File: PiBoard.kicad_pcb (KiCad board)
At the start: 4 copper layers, 90.1 x 92.5 mm, 129 parts, among them IC1 TCAN337DCNR, IC2 TPS2557QDRBTQ1, IC3 LM74502HDDFR, IC4 AP64501QSP-13, IC5 TPS2557QDRBTQ1, IC7 TPS2557QDRBTQ1, IC8 TPS2557QDRBTQ1, J1 CarLVPowerConnector, J10 USB_C_Receptacle, J11 RTC Battery Port, J14 4x nano-fit, J2 Display Breakout, J3 2222, J5 USB_C_Receptacle_USB2.0_16P, J6 CarCANConnector, J7 USB_C_Receptacle_USB2.0_16P, J8 CarCANConnector, J9 HDMI_E, Q1 PSMN8R5-40MSDX, SW1 SW_Push, SW2 SW_Push, U13 CDSOT23-T24CAN, U14 MCP2515-E/STVAO, Y4 8 MHz

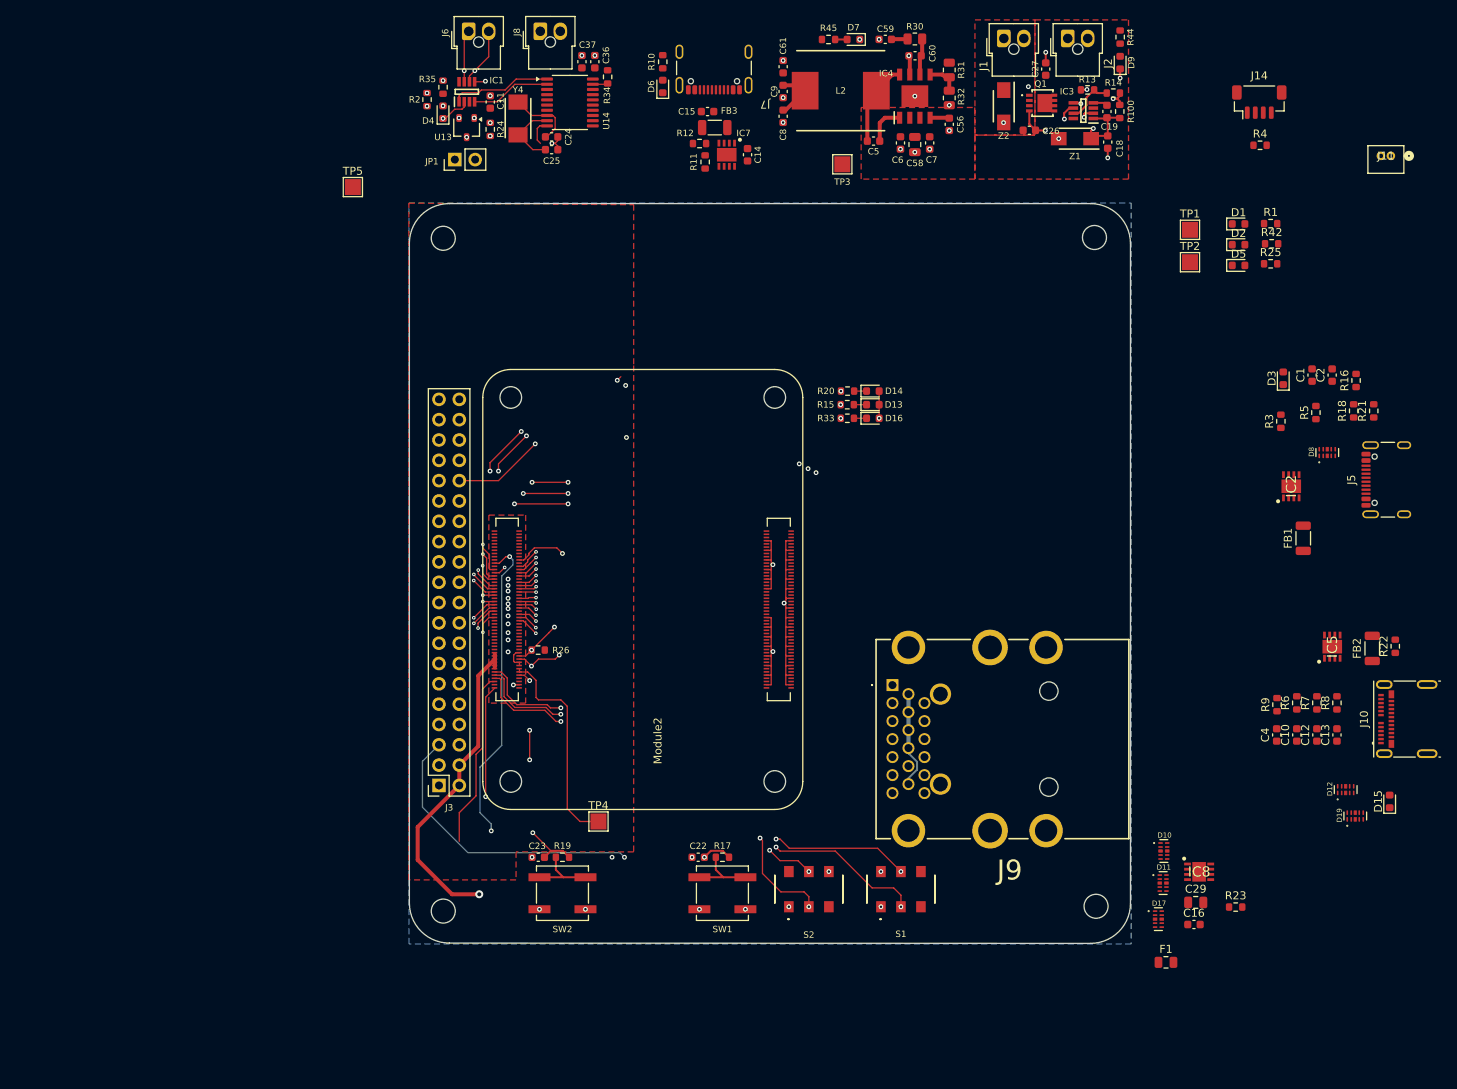
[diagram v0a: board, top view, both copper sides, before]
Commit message: I hate my life
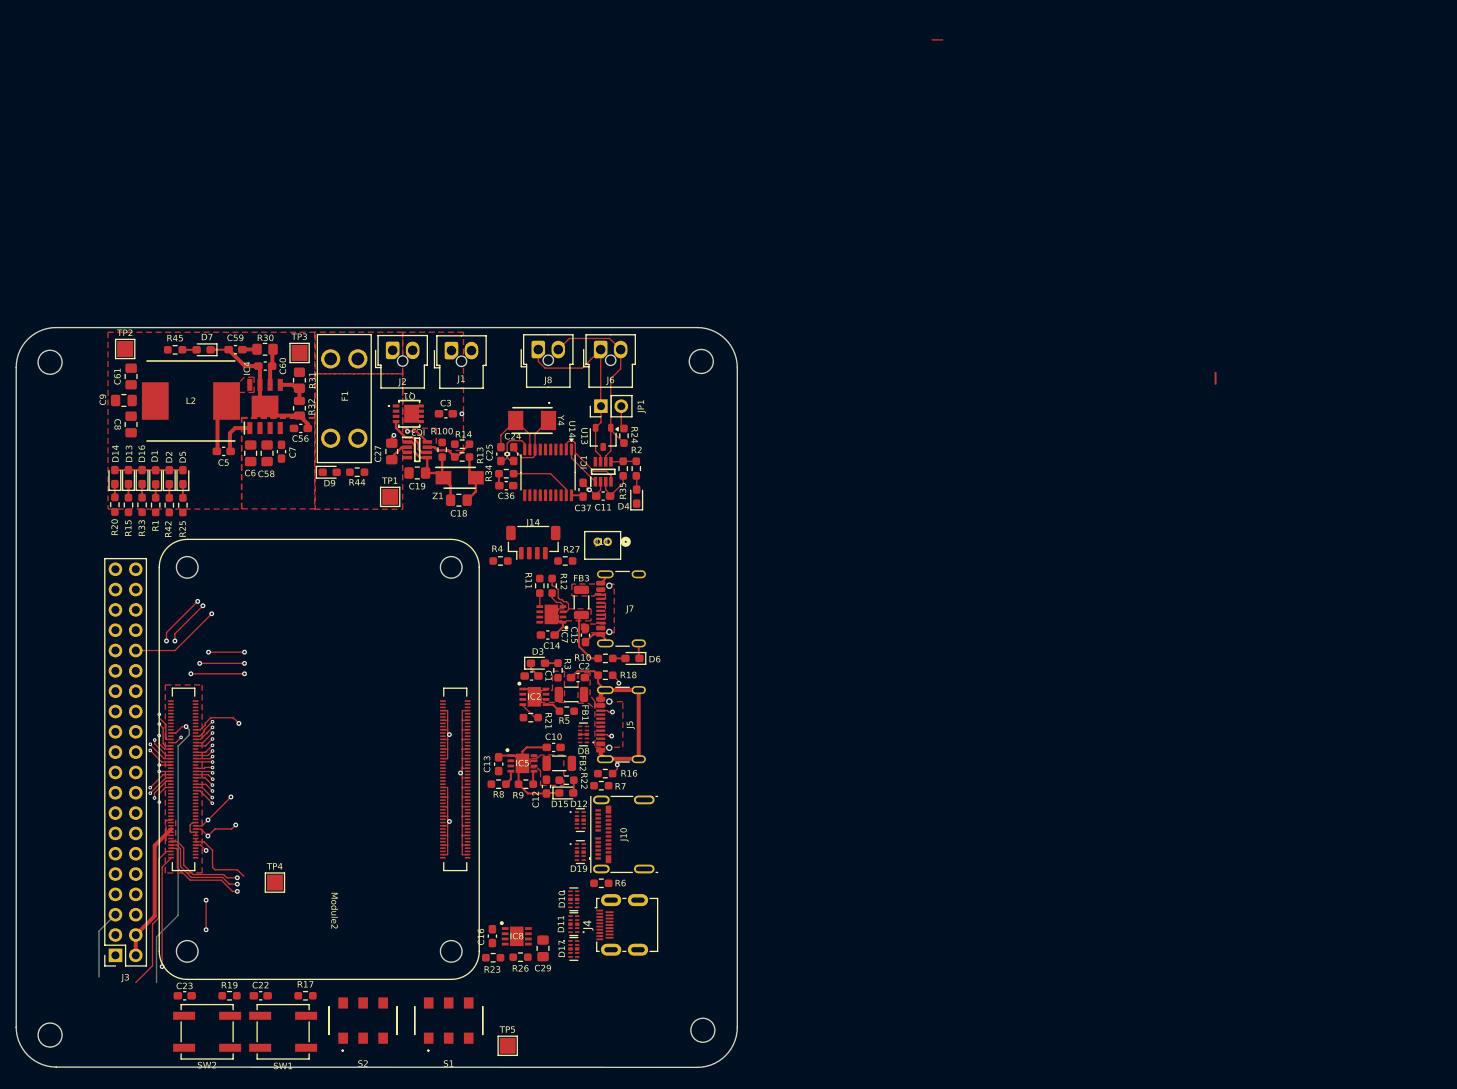
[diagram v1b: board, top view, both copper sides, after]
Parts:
- removed C26: 22n, Capacitor_SMD:C_0603_1608Metric
- removed C4: 120uF, Capacitor_SMD:C_0603_1608Metric
- removed J9: HDMI_E, Controls_Pi:MX50019NQ1
- removed Z2: SMAF4751A-TP, UTSVT_Passives:SODFL5026X125N
- added C3: 0.1u, Capacitor_SMD:C_0603_1608Metric_Pad1.08x0.95mm_HandSolder, F.Cu at (106.3, 77.5)
- added J4: HDMI_D_1.4, Connector_Video:HDMI_Micro-D_Molex_46765-1x01, F.Cu at (130.3, 141.4)
- added R27: 10K, Resistor_SMD:R_0603_1608Metric_Pad0.98x0.95mm_HandSolder, F.Cu at (121.3, 95.9)
- C1, C10, C11, C12, C13, C14, C15, C16, C2, C22, C23, C36, C37, C5, C56, C59, C60, C7: footprint Capacitor_SMD:C_0603_1608Metric -> Capacitor_SMD:C_0603_1608Metric_Pad1.08x0.95mm_HandSolder
- C18, C19, C27, C6, C61, C8, C9: footprint Capacitor_SMD:C_0603_1608Metric -> Capacitor_SMD:C_0805_2012Metric_Pad1.18x1.45mm_HandSolder
- C24, C25: value 26 pF -> 22 pF; footprint Capacitor_SMD:C_0603_1608Metric -> Capacitor_SMD:C_0603_1608Metric_Pad1.08x0.95mm_HandSolder
- C29, C58: footprint Capacitor_SMD:C_0805_2012Metric -> Capacitor_SMD:C_0805_2012Metric_Pad1.18x1.45mm_HandSolder
- D1, D13, D14, D15, D16, D2, D3, D4, D5, D6, D7, D9: footprint LED_SMD:LED_0603_1608Metric -> LED_SMD:LED_0603_1608Metric_Pad1.05x0.95mm_HandSolder
- F1: value 1A -> 3568; footprint Fuse:Fuse_0805_2012Metric -> Controls_Pi:FUSE_3568
- Q1: footprint UTSVT_Power_SP:PSMN8R5-40MSDX -> UTSVT_Power:PSMN8R5-40MSDX
- R1, R42: value 1k -> 700; footprint Resistor_SMD:R_0603_1608Metric -> Resistor_SMD:R_0603_1608Metric_Pad0.98x0.95mm_HandSolder
- R10, R100, R11, R12, R13, R14, R15, R16, R17, R18, R19, R2, R20, R21, R22, R23, R24, R25, R26, R3, R33, R34, R35, R44, R45, R5, R6, R7, R8, R9: footprint Resistor_SMD:R_0603_1608Metric -> Resistor_SMD:R_0603_1608Metric_Pad0.98x0.95mm_HandSolder
- R30, R31: footprint Resistor_SMD:R_0805_2012Metric -> Resistor_SMD:R_0805_2012Metric_Pad1.20x1.40mm_HandSolder
- R4: value 10K 1% -> 10K; footprint Resistor_SMD:R_0603_1608Metric -> Resistor_SMD:R_0603_1608Metric_Pad0.98x0.95mm_HandSolder
- moved R1 143.7 mm to (70.1, 89.0), turned to -90 degrees
- moved R42 141.6 mm to (71.8, 89.0), turned to -90 degrees
- moved R25 139.3 mm to (73.5, 89.0), turned to -90 degrees
- moved D1 139.0 mm to (70.1, 85.5), turned to 90 degrees
- moved D2 136.8 mm to (71.8, 85.5), turned to 90 degrees
- moved D5 134.6 mm to (73.5, 85.5), turned to 90 degrees
- moved TP2 133.5 mm to (66.2, 69.4)
- moved F1 124.6 mm to (93.6, 75.6), turned to -90 degrees
- moved R21 112.1 mm to (116.9, 115.5), turned to 0 degrees
- moved D9 111.3 mm to (91.8, 84.8), turned to 0 degrees
- moved R44 109.8 mm to (95.2, 84.8), turned to 180 degrees
- moved J11 109.1 mm to (126.6, 93.5)
- moved TP5 109.1 mm to (114.1, 156.5)
- moved R4 108.2 mm to (113.2, 95.9), turned to 180 degrees
- moved J14 106.1 mm to (117.3, 93.6)
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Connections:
- D11 pad 1: /High Speed/HDMI0_CK_P -> /High Speed/HDMI0_CK_N
- D11 pad 10: /High Speed/HDMI0_CK_P -> /High Speed/HDMI0_CK_N
- D11 pad 2: /High Speed/HDMI0_CK_N -> /High Speed/HDMI0_CK_P
- D11 pad 4: /High Speed/HDMI0_D1_P -> /High Speed/HDMI0_D1_N
- D11 pad 5: /High Speed/HDMI0_D1_N -> /High Speed/HDMI0_D1_P
- D11 pad 6: /High Speed/HDMI0_D1_N -> /High Speed/HDMI0_D1_P
- D11 pad 7: /High Speed/HDMI0_D1_P -> /High Speed/HDMI0_D1_N
- D11 pad 9: /High Speed/HDMI0_CK_N -> /High Speed/HDMI0_CK_P
- D12 pad 1: /High Speed/USB_HUB_D- -> unconnected-(D12-D1+-Pad1)
- D12 pad 10: /High Speed/USB_HUB_D- -> unconnected-(D12-NC_4-Pad10)
- D12 pad 2: /High Speed/USB_HUB_D+ -> unconnected-(D12-D1--Pad2)
- D12 pad 4: unconnected-(D12-D2+-Pad4) -> /High Speed/USB_HUB_D-
- D12 pad 5: unconnected-(D12-D2--Pad5) -> /High Speed/USB_HUB_D+
- D12 pad 6: unconnected-(D12-NC_1-Pad6) -> /High Speed/USB_HUB_D+
- D12 pad 7: unconnected-(D12-NC_2-Pad7) -> /High Speed/USB_HUB_D-
- D12 pad 9: /High Speed/USB_HUB_D+ -> unconnected-(D12-NC_3-Pad9)
- D17 pad 2: /High Speed/HDMI0_HOTPLUG -> /High Speed/HDMI0_SCL
- D17 pad 4: /High Speed/HDMI0_SCL -> /High Speed/HDMI0_SDA
- D17 pad 5: /High Speed/HDMI0_SDA -> /High Speed/HDMI0_HOTPLUG
- D17 pad 6: /High Speed/HDMI0_SDA -> /High Speed/HDMI0_HOTPLUG
- D17 pad 7: /High Speed/HDMI0_SCL -> /High Speed/HDMI0_SDA
- D17 pad 9: /High Speed/HDMI0_HOTPLUG -> /High Speed/HDMI0_SCL
- D8 pad 1: /High Speed/USB_DBG_D- -> unconnected-(D8-D1+-Pad1)
- D8 pad 10: /High Speed/USB_DBG_D- -> unconnected-(D8-NC_4-Pad10)
- D8 pad 2: /High Speed/USB_DBG_D+ -> unconnected-(D8-D1--Pad2)
- D8 pad 4: unconnected-(D8-D2+-Pad4) -> /High Speed/USB_DBG_D-
- D8 pad 5: unconnected-(D8-D2--Pad5) -> /High Speed/USB_DBG_D+
- D8 pad 6: unconnected-(D8-NC_1-Pad6) -> /High Speed/USB_DBG_D+
- D8 pad 7: unconnected-(D8-NC_2-Pad7) -> /High Speed/USB_DBG_D-
- D8 pad 9: /High Speed/USB_DBG_D+ -> unconnected-(D8-NC_3-Pad9)
- Q1 pad 1: /Power Distribution/LV+ -> +24V
- Q1 pad 10: +24V -> /Power Distribution/LV+
- Q1 pad 11: +24V -> /Power Distribution/LV+
- Q1 pad 2: /Power Distribution/LV+ -> +24V
- Q1 pad 3: /Power Distribution/LV+ -> +24V
- Q1 pad 5: +24V -> /Power Distribution/LV+
- Q1 pad 6: +24V -> /Power Distribution/LV+
- Q1 pad 7: +24V -> /Power Distribution/LV+
- Q1 pad 8: +24V -> /Power Distribution/LV+
- Q1 pad 9: +24V -> /Power Distribution/LV+
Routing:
- net /CM5 GPIO/EEPROM_nWP: track 77.9 -> 8.60 mm, vias 3 -> 1
- net /CM5 GPIO/BT_Disable: track 73.6 -> 11.6 mm, vias 3 -> 1
- net /CM5 GPIO/WiFi_Disable: track 71.8 -> 11.4 mm, vias 3 -> 1
- net /CM5 GPIO/nRPIBOOT: track 59.2 -> 11.8 mm, vias 3 -> 1
- net /CM5 GPIO/GPIO13: track 91.1 -> 50.0 mm, vias 5 -> 3
- net /CM5 GPIO/GPIO19: track 87.5 -> 46.6 mm, vias 5 -> 3
- net /CM5 GPIO/GPIO26: track 84.3 -> 43.6 mm, vias 5 -> 3
- net unconnected-(Module2A-SDA0-Pad82): track 64.7 -> 29.1 mm
- net /CM5 GPIO/PWR_BUTT: track 47.1 -> 12.9 mm, vias 4 -> 3
- net +5V: track 47.0 -> 17.6 mm, vias 1 -> 0
- net /CM5 GPIO/GPIO3: track 79.1 -> 51.3 mm, vias 2 -> 1
- net unconnected-(Module2A-SCL0-Pad80): track 0.00 -> 24.8 mm, vias 0 -> 2
- net +3.3V: track 39.2 -> 19.6 mm, vias 2 -> 0
- net /CM5 GPIO/CAN_SPI_CS: track 43.5 -> 26.1 mm
- net +1.8V: track 26.8 -> 9.40 mm
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- added copper zone on F.Cu, net +5V
- added copper zone on F.Cu, net /High Speed/USB-C/VBUS_DBG
- added copper zone on F.Cu, net /High Speed/USB-C/VBUS_HUB
- added copper zone on F.Cu, net /High Speed/USB-C/VBUS_PWR
- added copper zone on F.Cu, net Net-(C15-Pad1)
- added copper zone on F.Cu, net Net-(C2-Pad1)
- added copper zone on F.Cu, net Net-(IC4-SW)
- added copper zone on F.Cu, net Net-(J2-+24V)
- removed copper zone on F.Cu, net +3.3V
- removed copper zone on B.Cu, net GND
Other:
- board text added: "For Instructional Use Only."
- board text added: "SOLIDWORKS Educational Product."
- board text removed: "Left some of these pwr components 0805 (?)"
- board text removed: "Trying to keep this space more open for fancy routing ig"

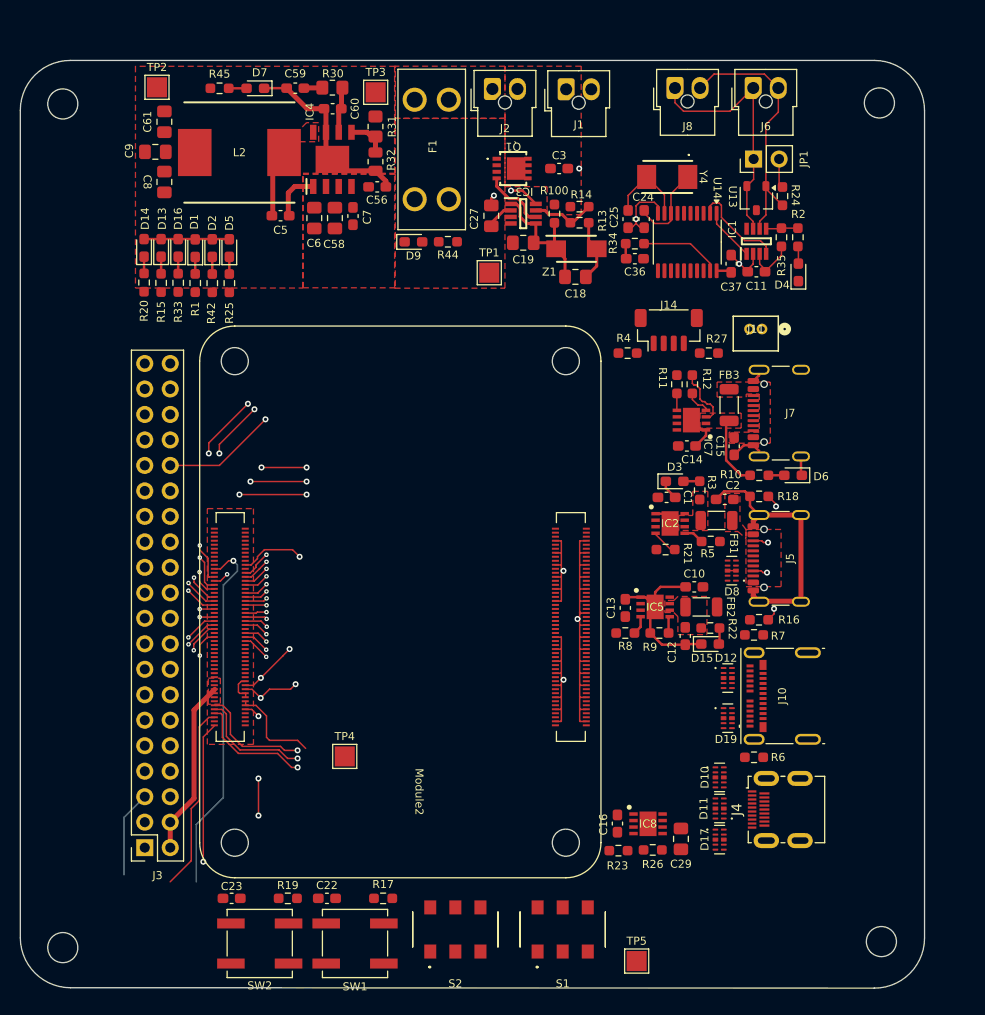
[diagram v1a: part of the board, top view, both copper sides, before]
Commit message: I'm unhappy with the state of the world
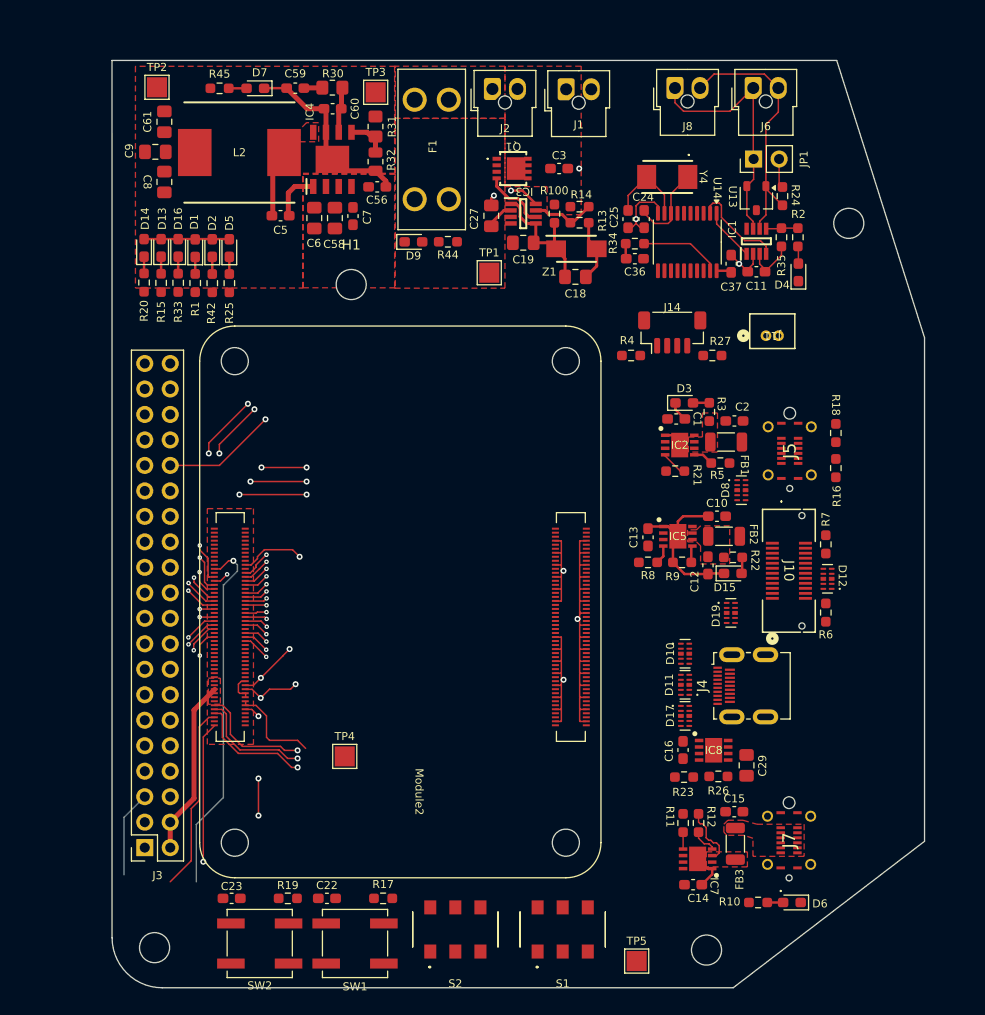
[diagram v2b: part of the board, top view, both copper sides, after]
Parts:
- J10: footprint Connector_USB:USB_C_Receptacle_Molex_105450-0101 -> Controls_Pi:CONN_221608-0001_MOL
- J5: footprint Connector_USB:USB_C_Receptacle_GCT_USB4105-xx-A_16P_TopMnt_Horizontal -> Controls_Pi:2193200001
- J7: footprint UTSVT_Connectors:USB_C_Receptacle_GCT_USB4105-xx-A_16P_TopMnt_Horizontal -> Controls_Pi:2193200001
- moved C14 43.7 mm to (119.7, 148.9)
- moved R11 43.7 mm to (118.7, 142.8)
- moved R12 43.7 mm to (120.2, 142.8)
- moved FB3 43.7 mm to (123.9, 144.8)
- moved IC7 43.7 mm to (120.1, 146.3)
- moved J7 42.6 mm to (129.2, 144.5)
- moved D6 42.6 mm to (129.5, 150.7)
- moved R10 42.6 mm to (126.2, 150.7)
- moved C15 36.4 mm to (123.8, 141.7), turned to 180 degrees
- moved H1 33.9 mm to (85.6, 89.1)
- moved H4 17.5 mm to (121.0, 155.4)
- moved R16 16.9 mm to (133.9, 107.4), turned to 90 degrees
- moved R6 16.1 mm to (132.9, 121.8), turned to -90 degrees
- moved D12 14.0 mm to (133.1, 118.4), turned to 180 degrees
- moved D11 12.8 mm to (118.9, 129.0)
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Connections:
- D8 pad 1: unconnected-(D8-D1+-Pad1) -> /High Speed/USB_DBG_D-
- D8 pad 10: unconnected-(D8-NC_4-Pad10) -> /High Speed/USB_DBG_D-
- D8 pad 2: unconnected-(D8-D1--Pad2) -> /High Speed/USB_DBG_D+
- D8 pad 4: /High Speed/USB_DBG_D- -> unconnected-(D8-D2+-Pad4)
- D8 pad 5: /High Speed/USB_DBG_D+ -> unconnected-(D8-D2--Pad5)
- D8 pad 6: /High Speed/USB_DBG_D+ -> unconnected-(D8-NC_1-Pad6)
- D8 pad 7: /High Speed/USB_DBG_D- -> unconnected-(D8-NC_2-Pad7)
- D8 pad 9: unconnected-(D8-NC_3-Pad9) -> /High Speed/USB_DBG_D+
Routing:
- net GND: track 152.4 -> 118.8 mm
- net Net-(J5-CC2): track 6.86 -> 0.00 mm, vias 2 -> 0
- net Net-(J5-CC1): track 6.68 -> 0.00 mm, vias 2 -> 0
- net /High Speed/USB-C/VBUS_PWR: track 13.1 -> 6.44 mm
- removed copper zone on F.Cu, net Net-(C2-Pad1)
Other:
- board size 90.1 x 92.5 mm -> 81 x 92.4 mm
- board text added: "Fuckass constraints"
- board text added: "I mean what am I supposed to do here"
